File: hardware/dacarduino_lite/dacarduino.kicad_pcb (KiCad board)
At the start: 2 copper layers, 83 x 59 mm, 42 parts, among them J11 CV IN, J12 CV IN, J13 CV IN, J17 VCC, J18 Vin, J3 CV OUT A, J4 CV OUT B, J5 GATE OUT A, J7 GATE IN, Q1 2N3904, Q3 2N3904, U1 MCP4922, U2 TL972

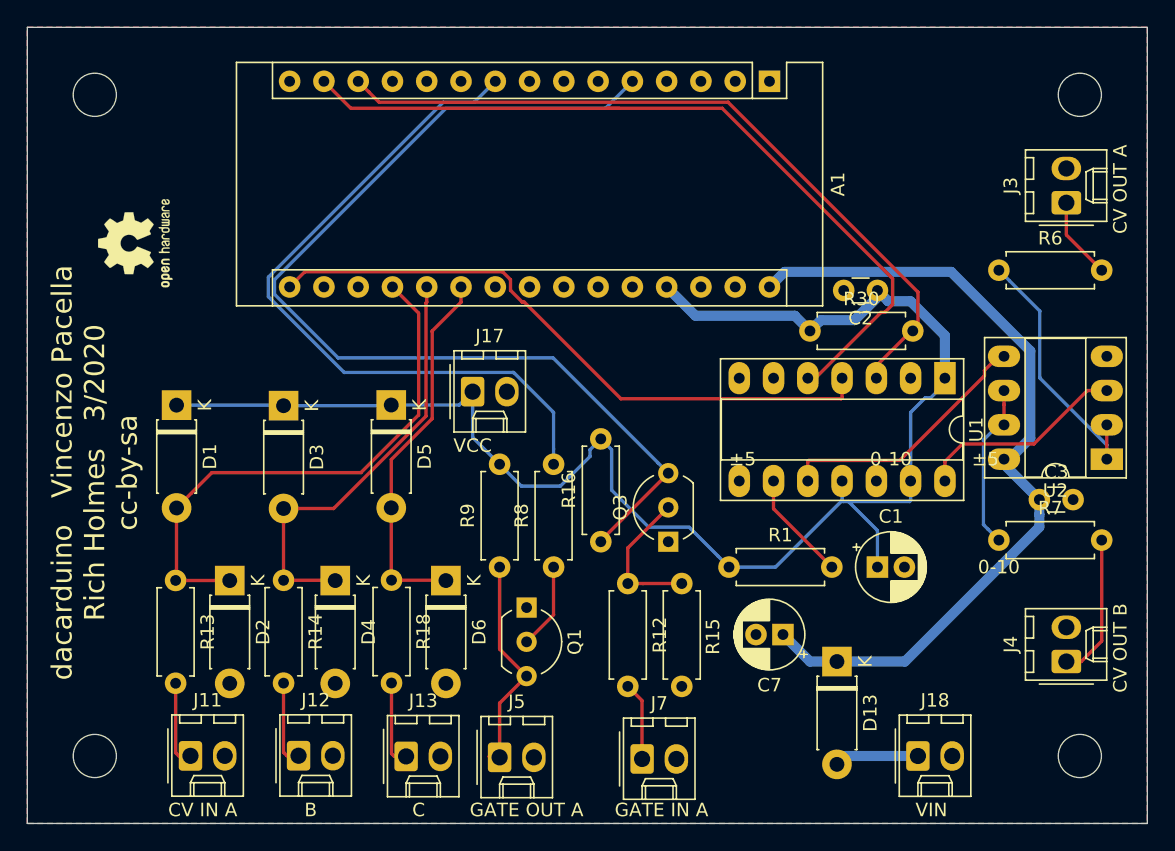
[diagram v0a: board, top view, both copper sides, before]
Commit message: Backlog of many changes
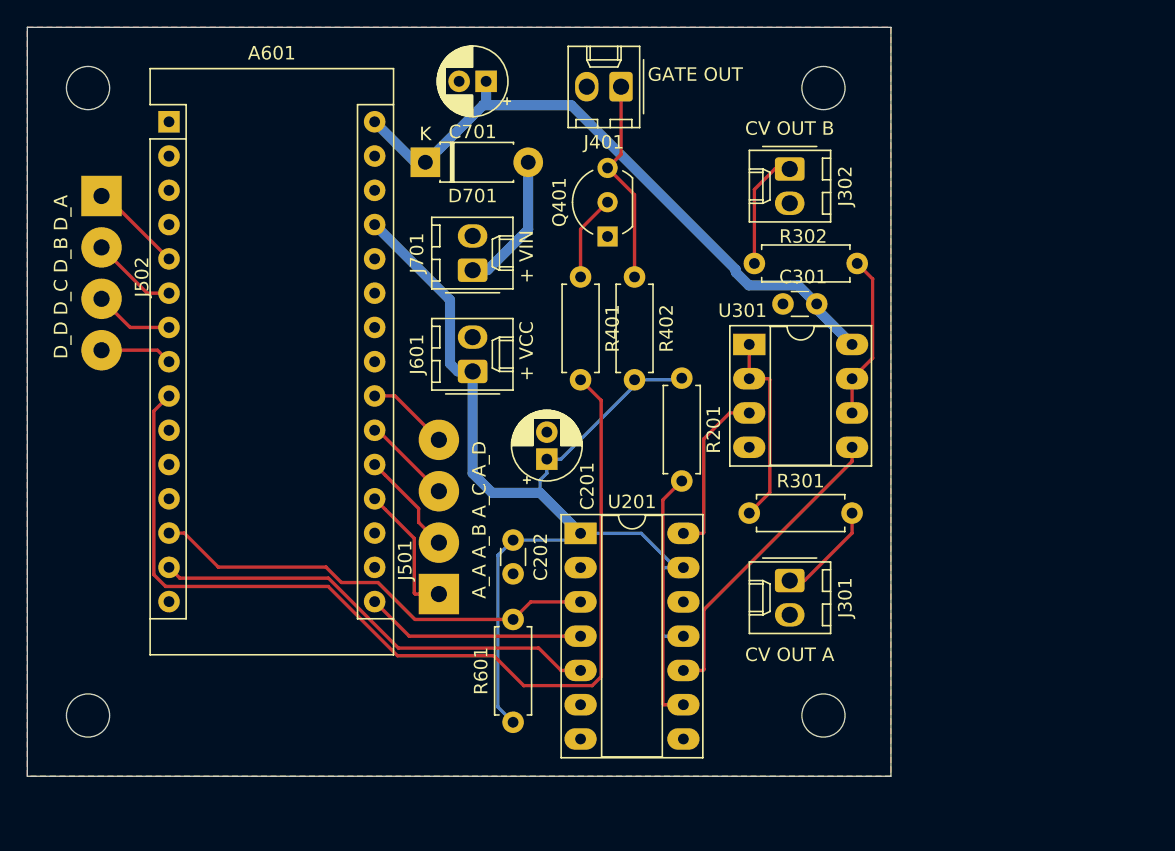
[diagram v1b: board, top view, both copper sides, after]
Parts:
- removed D1, D2, D3, D4, D5, D6: 1N5817, Diode_THT:D_DO-41_SOD81_P7.62mm_Horizontal
- removed J11, J12, J13: CV IN, Connector_Molex:Molex_KK-254_AE-6410-02A_1x02_P2.54mm_Vertical
- removed J7: GATE IN, Connector_Molex:Molex_KK-254_AE-6410-02A_1x02_P2.54mm_Vertical
- removed Q3: 2N3904, Package_TO_SOT_THT:TO-92_Inline_Wide
- removed R12: 100k, Resistor_THT:R_Axial_DIN0207_L6.3mm_D2.5mm_P7.62mm_Horizontal
- removed R13, R14, R18: 1k, Resistor_THT:R_Axial_DIN0207_L6.3mm_D2.5mm_P7.62mm_Horizontal
- removed R15: 1M, Resistor_THT:R_Axial_DIN0207_L6.3mm_D2.5mm_P7.62mm_Horizontal
- removed R16: 10k, Resistor_THT:R_Axial_DIN0207_L6.3mm_D2.5mm_P7.62mm_Horizontal
- removed REF**: OSHW-Logo2_7.3x6mm_SilkScreen, Symbol:OSHW-Logo2_7.3x6mm_SilkScreen
- added J501: Conn_01x04, Connector_Wire:SolderWirePad_1x04_P3.81mm_Drill1.2mm, F.Cu at (155.5, 135.0)
- added J502: Conn_01x04, Connector_Wire:SolderWirePad_1x04_P3.81mm_Drill1.2mm, F.Cu at (130.5, 105.5)
- U301: renamed from U2; value TL972 -> MCP6002
- moved H104 53.0 mm to (184.0, 97.5), turned to 180 degrees
- moved J401 50.5 mm to (169.0, 97.4), turned to 180 degrees
- moved H103 49.8 mm to (184.0, 144.0), turned to 180 degrees
- moved J701 48.8 mm to (158.0, 111.0), turned to 90 degrees
- moved D701 48.0 mm to (154.5, 103.0), turned to 0 degrees
- moved C701 46.5 mm to (159.0, 97.0)
- moved A601 44.6 mm to (135.5, 100.0), turned to 0 degrees
- moved J302 41.9 mm to (181.5, 103.5), turned to 270 degrees
- moved R601 36.4 mm to (161.0, 144.5), turned to 90 degrees
- moved J301 34.7 mm to (181.5, 134.0), turned to 270 degrees
- moved C202 32.7 mm to (161.0, 131.0), turned to 270 degrees
- moved U201 29.3 mm to (166.0, 130.5), turned to 0 degrees
- moved Q401 28.1 mm to (168.0, 108.5), turned to 90 degrees
- moved U301 27.8 mm to (178.5, 116.5), turned to 0 degrees
- moved R301 25.8 mm to (178.5, 129.0)
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- renumbered A1 to A601, C1 to C201, C2 to C202, C3 to C301, C7 to C701, D13 to D701, H1 to H101, H2 to H102, H3 to H103, H4 to H104, J3 to J301, J4 to J302, J5 to J401, J17 to J601, J18 to J701, Q1 to Q401, R1 to R201, R6 to R301, R7 to R302, R8 to R401, R9 to R402, R30 to R601, U1 to U201
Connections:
- net +12V renamed +VIN
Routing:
- net /Arduino/D_IN_A: track 75.5 -> 6.93 mm
- net VCC: track 115.4 -> 83.7 mm
- net /Arduino/SCK: track 47.2 -> 16.3 mm
- net /Arduino/A_IN_A: track 40.5 -> 10.1 mm
- net /Arduino/MOSI: track 59.5 -> 33.7 mm
- net /Arduino/A_IN_B: track 32.1 -> 7.76 mm
- net /Arduino/DAC_CS: track 55.6 -> 33.7 mm
- net /Arduino/A_IN_C: track 27.9 -> 6.63 mm
- net /Arduino/D_OUT_A: track 52.8 -> 73.2 mm
- net +VIN: track 61.6 -> 47.9 mm
- net Net-(Q3-Pad2): track 10.9 -> 0.00 mm
- net Net-(R201-Pad2): track 8.87 -> 18.6 mm
- net /Arduino/D_IN_B: track 0.00 -> 6.40 mm
- net /Inputs/CV in C/CV_IN: track 6.40 -> 0.00 mm
- net /Inputs/CV in B/CV_IN: track 6.35 -> 0.00 mm
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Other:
- board size 83 x 59 mm -> 64 x 55.5 mm
- board text added: "+ VCC"
- board text added: "+ VIN"
- board text added: "A_A A_B A_C A_D"
- board text added: "D_D D_C D_B D_A"
- board text added: "GATE OUT"
- board text removed: "0-10"
- board text removed: "B"
- board text removed: "C"
- board text removed: "CV IN A"
- board text removed: "GATE IN A"
- board text removed: "GATE OUT A"
- board text removed: "VCC"
- board text removed: "VIN"
- board text removed: "±5"
